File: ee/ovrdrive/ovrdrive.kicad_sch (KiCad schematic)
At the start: 43 parts, among them J1 USB_A, J3 AVR-ISP-6, U1 SM3257ENT, U2 FLASH, U3 ATtiny24A-MM, U4 SN74LVC1G32DCKR, U5 DRV8837C

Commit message: Added BOM commmited leftover stuff.
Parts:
- R1, R2: MPN (none) -> RC0402FR-071ML
- U5: MPN (none) -> DRV8837CDSGR
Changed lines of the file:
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@@
       (effects (font (size 1.27 1.27)) hide)
     )
-    (property "MPN" "" (at 62.23 176.53 90)
+    (property "MPN" "RC0402FR-071ML" (at 62.23 176.53 90)
       (effects (font (size 1.27 1.27)) hide)
     )
@@
       (effects (font (size 1.27 1.27)) hide)
     )
-    (property "MPN" "" (at 33.655 176.53 90)
+    (property "MPN" "RC0402FR-071ML" (at 33.655 176.53 90)
       (effects (font (size 1.27 1.27)) hide)
     )
@@
       (effects (font (size 1.27 1.27)) hide)
     )
+    (property "MPN" "DRV8837CDSGR" (at 194.31 130.81 0)
+      (effects (font (size 1.27 1.27)) hide)
+    )

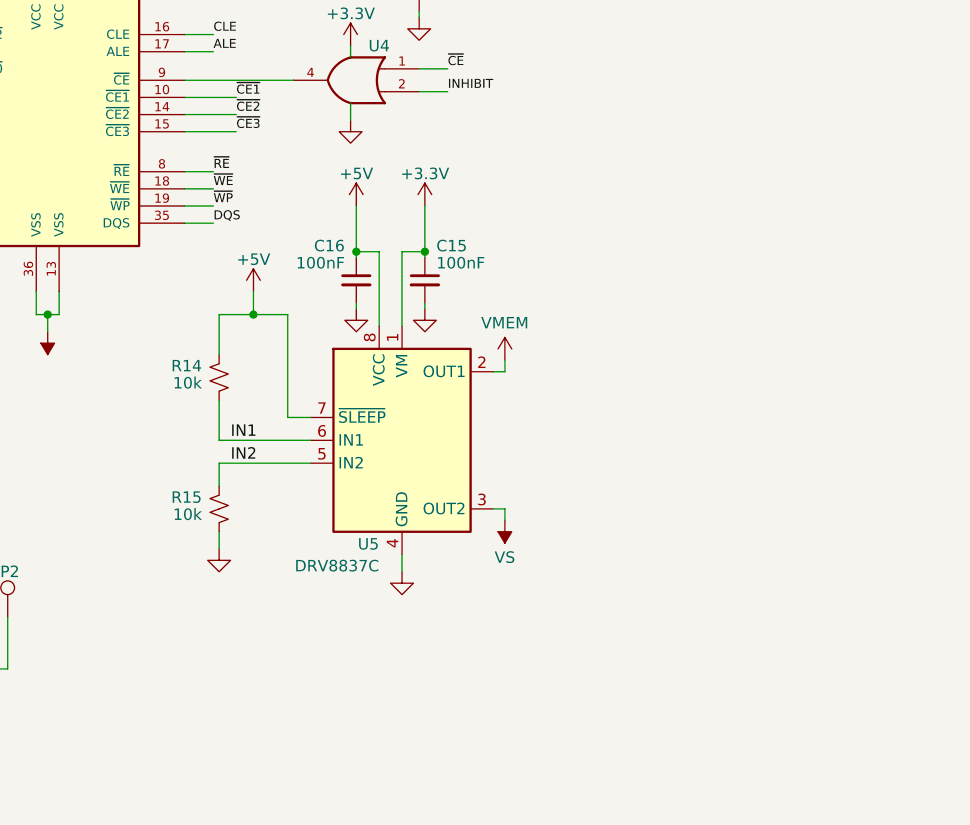
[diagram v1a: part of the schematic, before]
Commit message: Added license
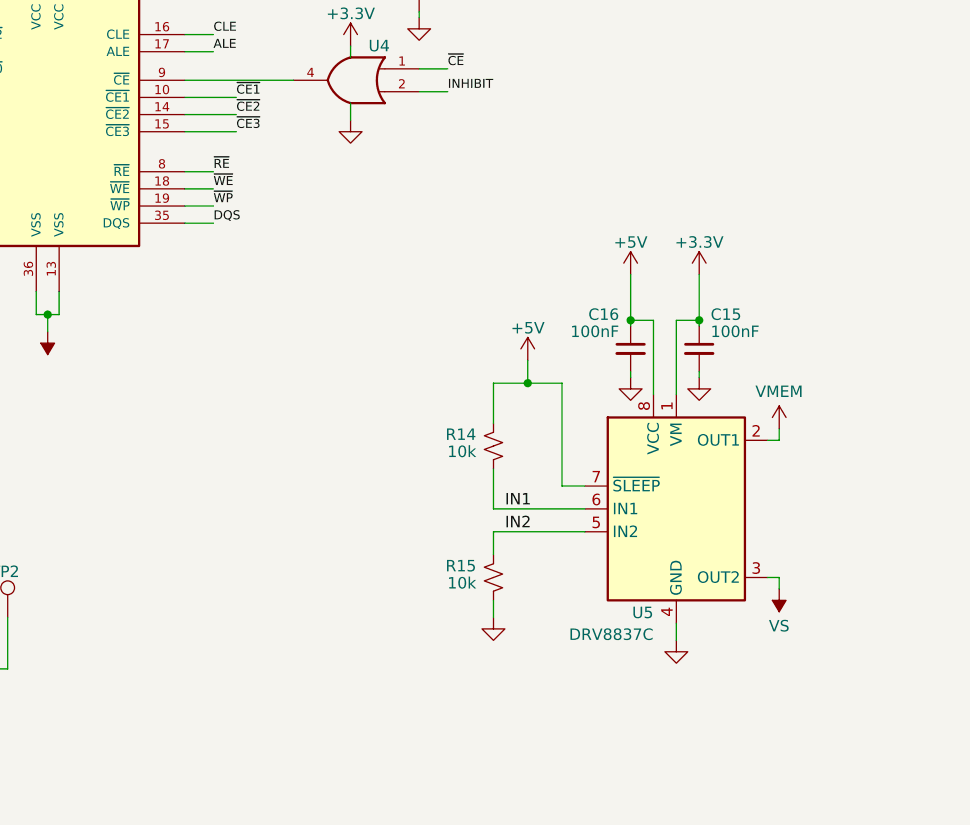
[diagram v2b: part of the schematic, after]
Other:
- moved on the sheet: C15, C16, R14, R15, U5
